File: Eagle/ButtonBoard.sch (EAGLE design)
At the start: 8 parts

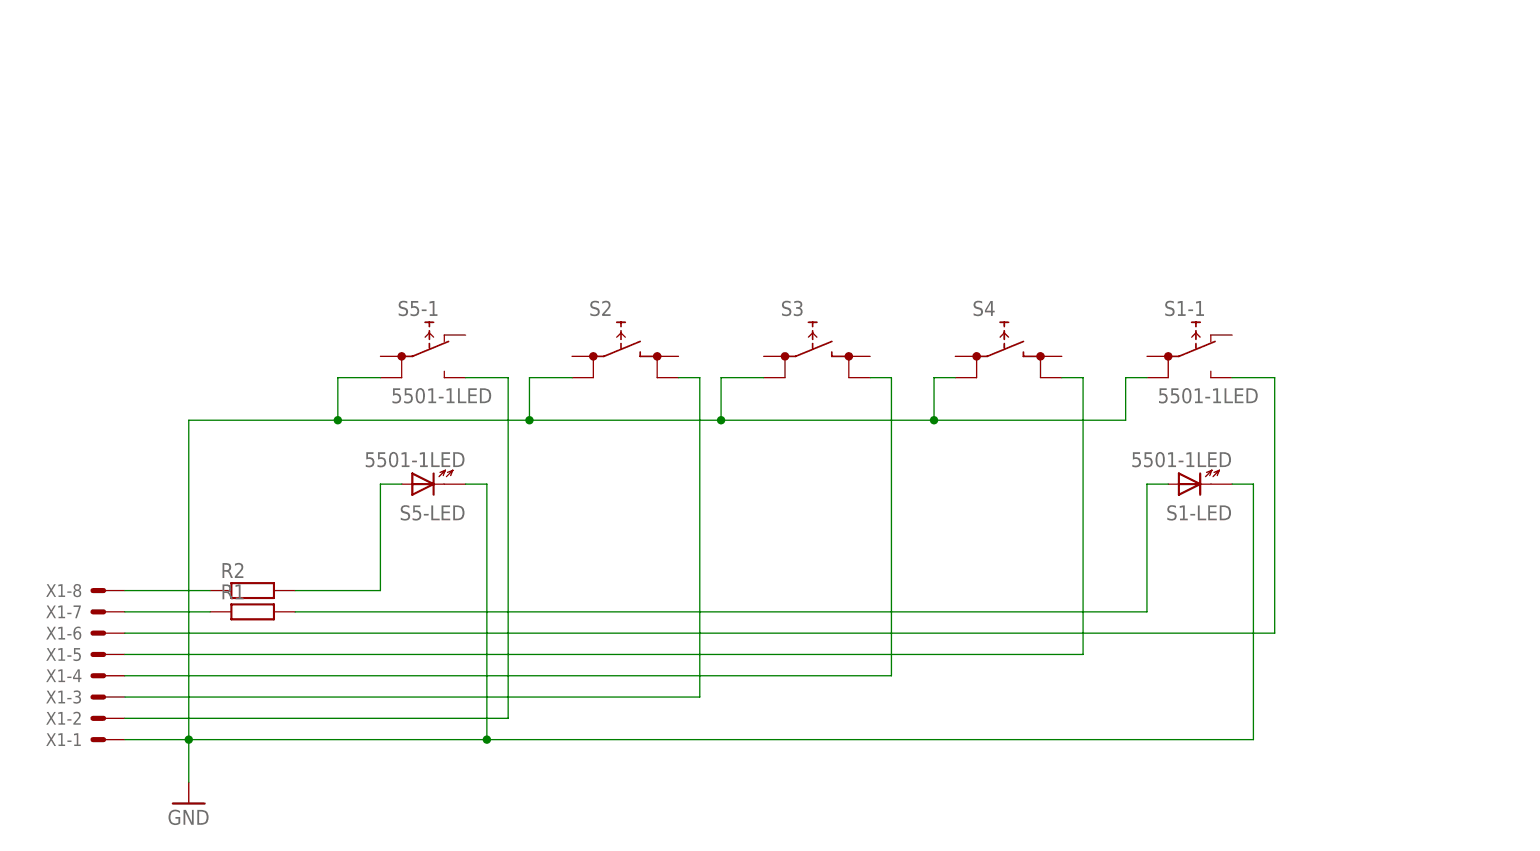
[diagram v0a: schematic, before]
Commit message: - some modifications, corrections, ...
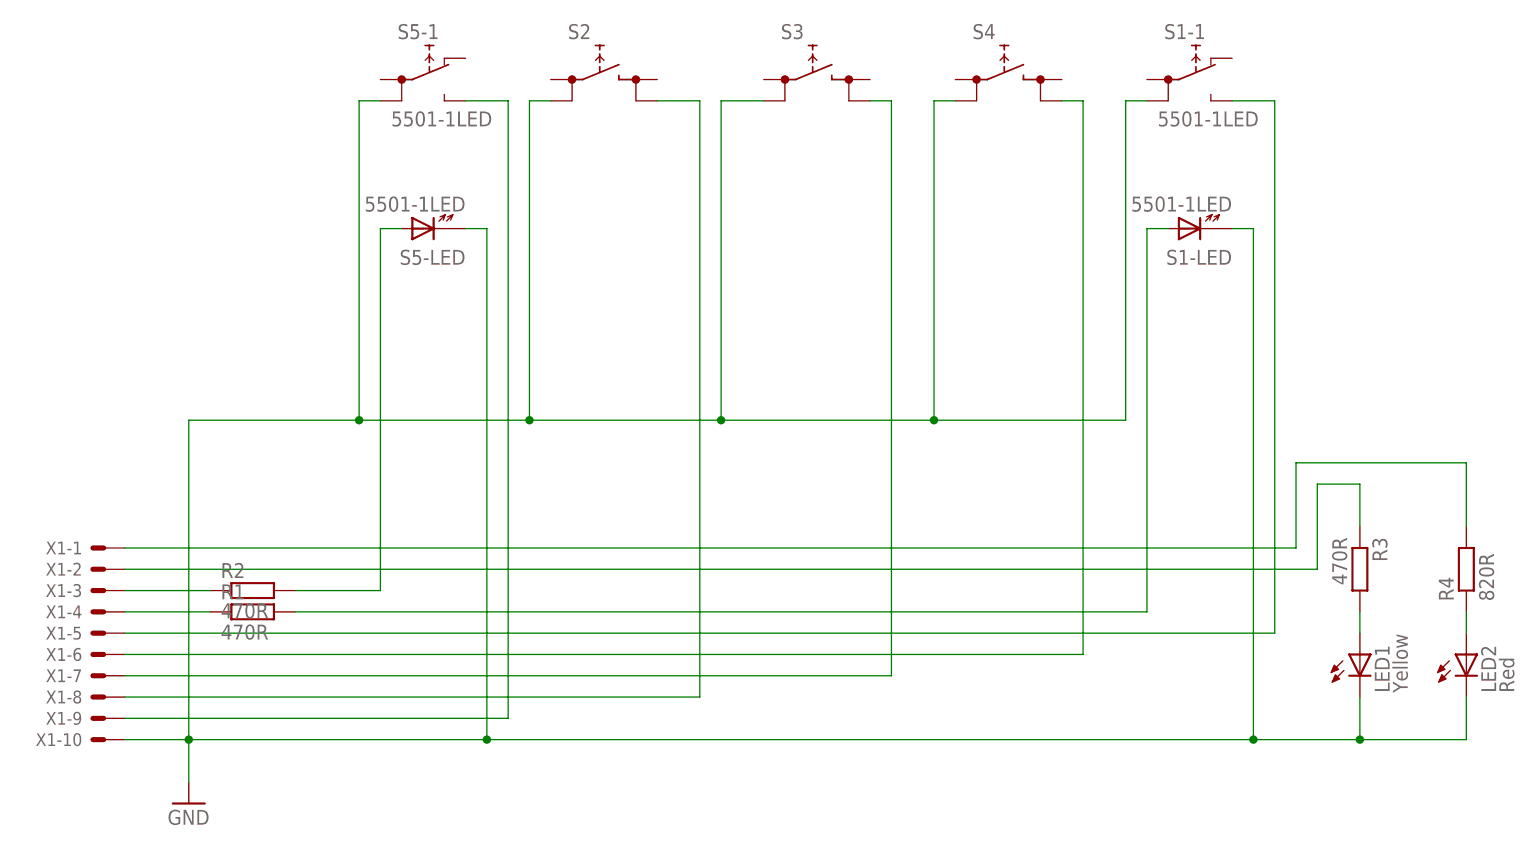
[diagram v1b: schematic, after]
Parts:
- added LED1: Yellow, led:LED3MM
- added LED2: Red, led:LED3MM
- added R3: 470R, rcl:R-EU_0207/10
- added R4: 820R, rcl:R-EU_0207/10
- R1, R2: value (none) -> 470R
- X1: device con-molex:KK-156-8 -> con-molex:KK-156-10
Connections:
- new net N$11: LED2.A, R4.1
- new net N$12: LED1.A, R3.2
- new net N$13: R3.1, X1-2.S
- new net N$14: R4.2, X1-1.S
- net GND: now also LED1.C, LED2.C, X1-10.S; no longer X1-1.S
- net N$2: now also X1-3.S; no longer X1-8.S
- net N$3: now also X1-4.S; no longer X1-7.S
- net N$4: now also X1-9.S; no longer X1-2.S
- net N$6: now also X1-8.S; no longer X1-3.S
- net N$7: now also X1-7.S; no longer X1-4.S
- net N$8: now also X1-6.S; no longer X1-5.S
- net N$9: now also X1-5.S; no longer X1-6.S
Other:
- moved on the sheet: S1-1, S1-LED, S2, S3, S4, S5-1, S5-LED, X1-1, X1-2, X1-3, X1-4, X1-5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
